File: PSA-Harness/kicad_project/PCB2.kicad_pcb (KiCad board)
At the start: 4 copper layers, 28.3 x 52.5 mm, 15 parts, among them J1 to_EPS_1, J2 to_EPS_2, J3 to_ESP_3, J7 USB_C_Receptacle, J8 B2B_1, J9 B2B_2, U1 DG419LEUA, U2 DG419LEUA

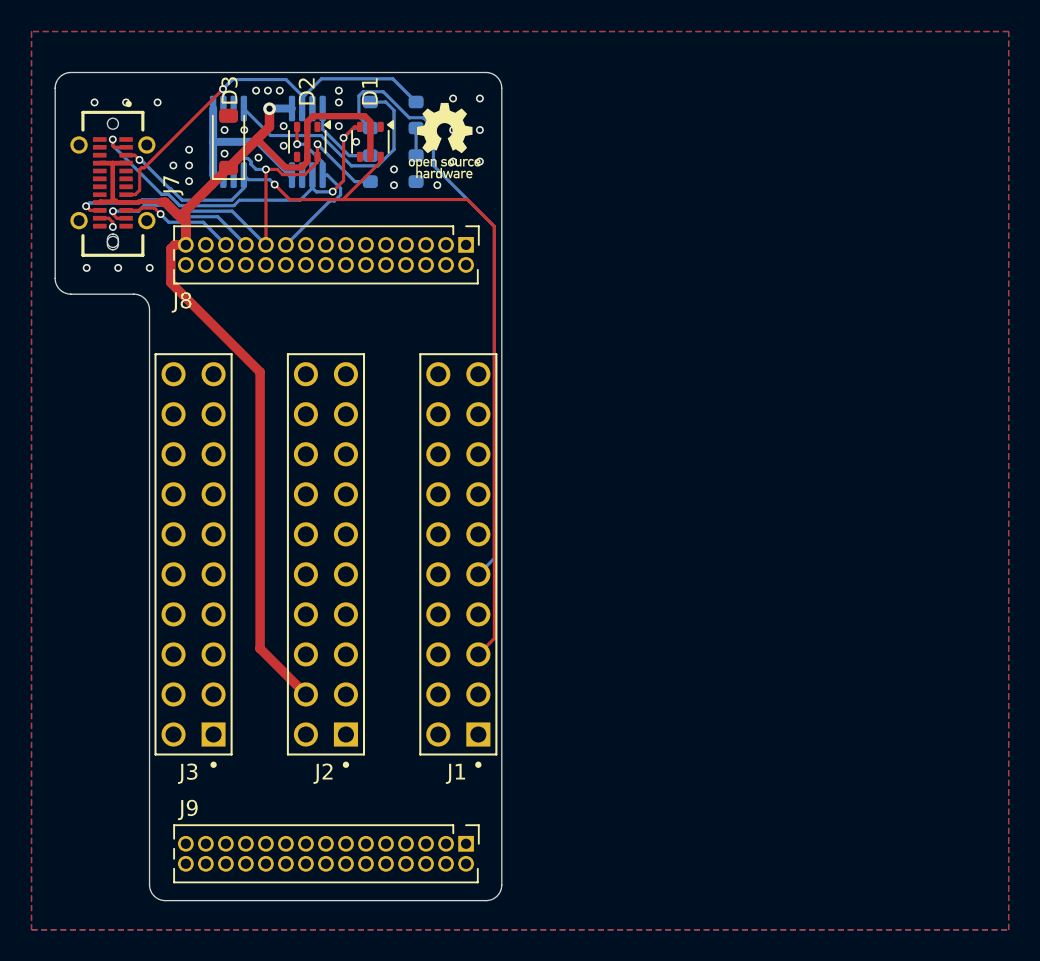
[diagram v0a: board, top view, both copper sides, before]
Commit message: PCB2 routed
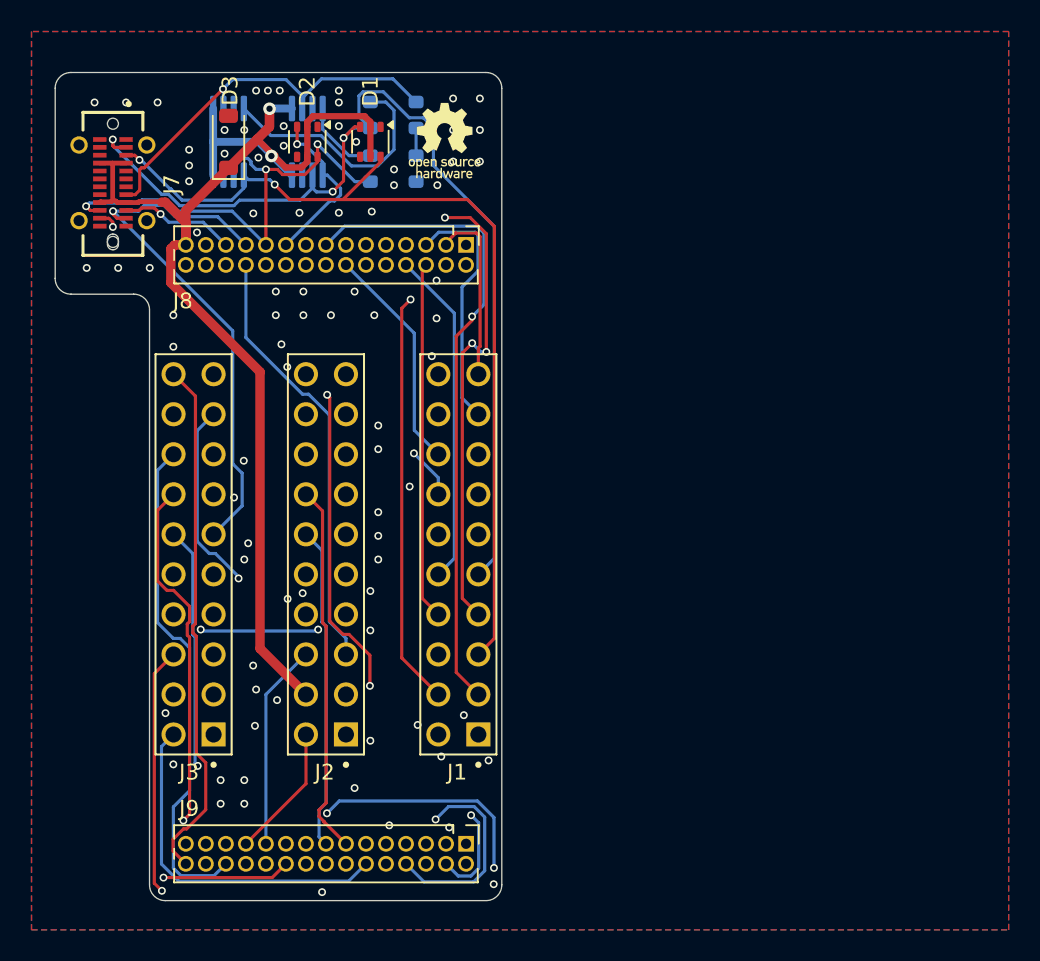
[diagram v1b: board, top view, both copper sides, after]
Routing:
- net 1: track 0.00 -> 52.2 mm, vias 0 -> 3
- net 50: track 0.00 -> 50.3 mm, vias 0 -> 2
- net 49: track 0.00 -> 48.8 mm, vias 0 -> 3
- net 54: track 0.00 -> 45.4 mm, vias 0 -> 4
- net 48: track 0.00 -> 43.2 mm, vias 0 -> 1
- net 2: track 0.00 -> 41.3 mm, vias 0 -> 1
- net 28: track 0.00 -> 38.1 mm, vias 0 -> 1
- net 30: track 0.00 -> 38.0 mm, vias 0 -> 1
- net 52: track 0.00 -> 37.6 mm, vias 0 -> 2
- net 47: track 0.00 -> 37.6 mm, vias 0 -> 1
- net 4: track 0.00 -> 36.6 mm, vias 0 -> 3
- net 40: track 0.00 -> 35.7 mm
- net 60: track 0.00 -> 33.4 mm
- net 21: track 0.00 -> 33.3 mm, vias 0 -> 1
- net 29: track 0.00 -> 33.0 mm, vias 0 -> 1
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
